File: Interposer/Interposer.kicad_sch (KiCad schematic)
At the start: 9 parts, among them J1 Cis_Electrode_In, J10 Trans_Electrode_Out, J11 Trans_Electrode_In, J2 Cis_Electrode_Out

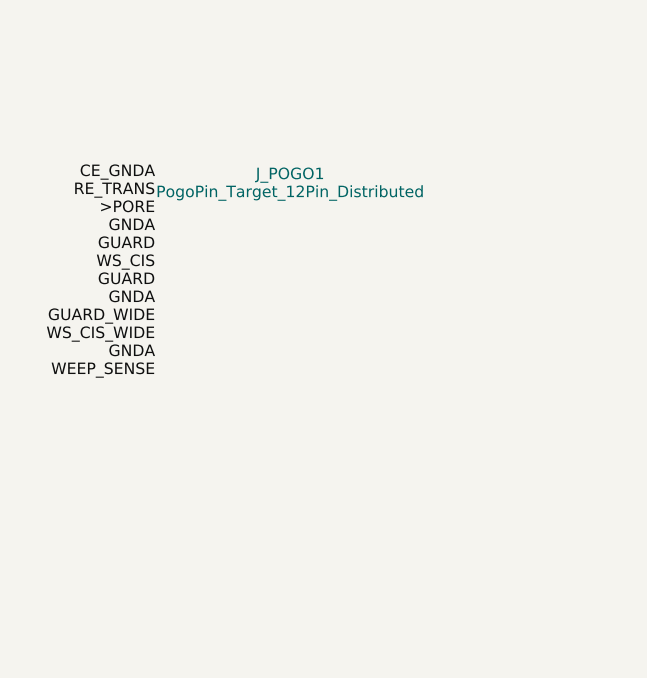
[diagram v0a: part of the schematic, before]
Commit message: adding new symbols
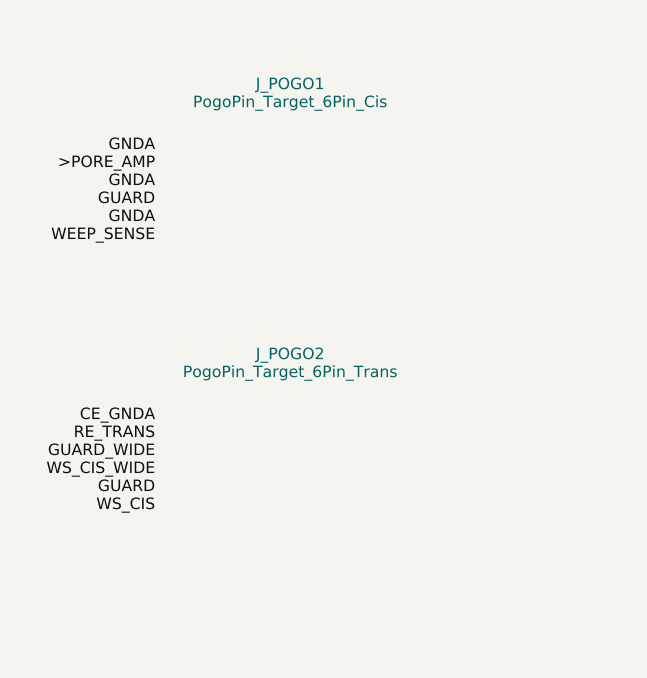
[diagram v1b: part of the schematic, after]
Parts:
- removed J_POGO1: PogoPin_Target_12Pin_Distributed, footprints:PogoPin_Target_12Pin_Distributed, symbol Connector_Generic:Conn_01x12
- added J_POGO1: PogoPin_Target_6Pin_Cis, footprints:PogoPin_Target_6Pin_Cis, symbol Connector_Generic:Conn_01x06
- added J_POGO2: PogoPin_Target_6Pin_Trans, footprints:PogoPin_Target_6Pin_Trans, symbol Connector_Generic:Conn_01x06
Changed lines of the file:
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@@
 		(comment 4 "Dual-Sided Ag/AgCl Ribbon Electrode Contacts with Weep Moat Leak Detection")
 	)
-	(symbol (lib_id "Connector_Generic:Conn_01x12") (at 70.0 80.0 0) (unit 1)
-		(property "Reference" "J_POGO1" (at 70.0 68.0 0) (effects (font (size 1.27 1.27))))
-		(property "Value" "PogoPin_Target_12Pin_Distributed" (at 70.0 70.0 0) (effects (font (size 1.27 1.27))))
-		(property "Footprint" "footprints:PogoPin_Target_12Pin_Distributed" (at 70.0 80.0 0) (hide yes) (effects (font (size 1.27 1.27))))
+	(symbol (lib_id "Connector_Generic:Conn_01x06") (at 70.0 70 0) (unit 1)
+		(property "Reference" "J_POGO1" (at 70.0 58 0) (effects (font (size 1.27 1.27))))
+		(property "Value" "PogoPin_Target_6Pin_Cis" (at 70.0 60 0) (effects (font (size 1.27 1.27))))
+		(property "Footprint" "footprints:PogoPin_Target_6Pin_Cis" (at 70.0 70 0) (hide yes) (effects (font (size 1.27 1.27))))
 		(pin "1")
 		(pin "2")
@@
 		(pin "5")
 		(pin "6")
-		(pin "7")
-		(pin "8")
-		(pin "9")
-		(pin "10")
-		(pin "11")
-		(pin "12")
+	)
+	(symbol (lib_id "Connector_Generic:Conn_01x06") (at 70.0 100 0) (unit 1)
+		(property "Reference" "J_POGO2" (at 70.0 88 0) (effects (font (size 1.27 1.27))))
+		(property "Value" "PogoPin_Target_6Pin_Trans" (at 70.0 90 0) (effects (font (size 1.27 1.27))))
+		(property "Footprint" "footprints:PogoPin_Target_6Pin_Trans" (at 70.0 100 0) (hide yes) (effects (font (size 1.27 1.27))))
+		(pin "1")
+		(pin "2")
+		(pin "3")
+		(pin "4")
+		(pin "5")
+		(pin "6")
 	)
 	(symbol (lib_id "Mechanical:MountingHole") (at 140.0 80.0 0) (unit 1)
@@
 		(pin "2")
 	)
-	(label "CE_GNDA" (at 55.0 68.0 180) (effects (font (size 1.27 1.27))))
-	(label "RE_TRANS" (at 55.0 70.0 180) (effects (font (size 1.27 1.27))))
-	(label ">PORE" (at 55.0 72.0 180) (effects (font (size 1.27 1.27))))
-	(label "GNDA" (at 55.0 74.0 180) (effects (font (size 1.27 1.27))))
-	(label "GUARD" (at 55.0 76.0 180) (effects (font (size 1.27 1.27))))
-	(label "WS_CIS" (at 55.0 78.0 180) (effects (font (size 1.27 1.27))))
-	(label "GUARD" (at 55.0 80.0 180) (effects (font (size 1.27 1.27))))
-	(label "GNDA" (at 55.0 82.0 180) (effects (font (size 1.27 1.27))))
-	(label "GUARD_WIDE" (at 55.0 84.0 180) (effects (font (size 1.27 1.27))))
-	(label "WS_CIS_WIDE" (at 55.0 86.0 180) (effects (font (size 1.27 1.27))))
-	(label "GNDA" (at 55.0 88.0 180) (effects (font (size 1.27 1.27))))
-	(label "WEEP_SENSE" (at 55.0 90.0 180) (effects (font (size 1.27 1.27))))
+	(label "GNDA" (at 55.0 65 180) (effects (font (size 1.27 1.27))))
+	(label ">PORE_AMP" (at 55.0 67 180) (effects (font (size 1.27 1.27))))
+	(label "GNDA" (at 55.0 69 180) (effects (font (size 1.27 1.27))))
+	(label "GUARD" (at 55.0 71 180) (effects (font (size 1.27 1.27))))
+	(label "GNDA" (at 55.0 73 180) (effects (font (size 1.27 1.27))))
+	(label "WEEP_SENSE" (at 55.0 75 180) (effects (font (size 1.27 1.27))))
+	(label "CE_GNDA" (at 55.0 95 180) (effects (font (size 1.27 1.27))))
+	(label "RE_TRANS" (at 55.0 97 180) (effects (font (size 1.27 1.27))))
+	(label "GUARD_WIDE" (at 55.0 99 180) (effects (font (size 1.27 1.27))))
+	(label "WS_CIS_WIDE" (at 55.0 101 180) (effects (font (size 1.27 1.27))))
+	(label "GUARD" (at 55.0 103 180) (effects (font (size 1.27 1.27))))
+	(label "WS_CIS" (at 55.0 105 180) (effects (font (size 1.27 1.27))))
 	(label ">PORE_AMP" (at 210.0 57.46 0) (effects (font (size 1.27 1.27))))
 	(label "GUARD" (at 210.0 60.0 0) (effects (font (size 1.27 1.27))))
